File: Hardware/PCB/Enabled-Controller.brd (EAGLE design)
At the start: 54 x 71 mm, 19 parts, among them J2 HEADER_FEMALE-1X2, J3 QWIIC, U1 ITSYBITSY

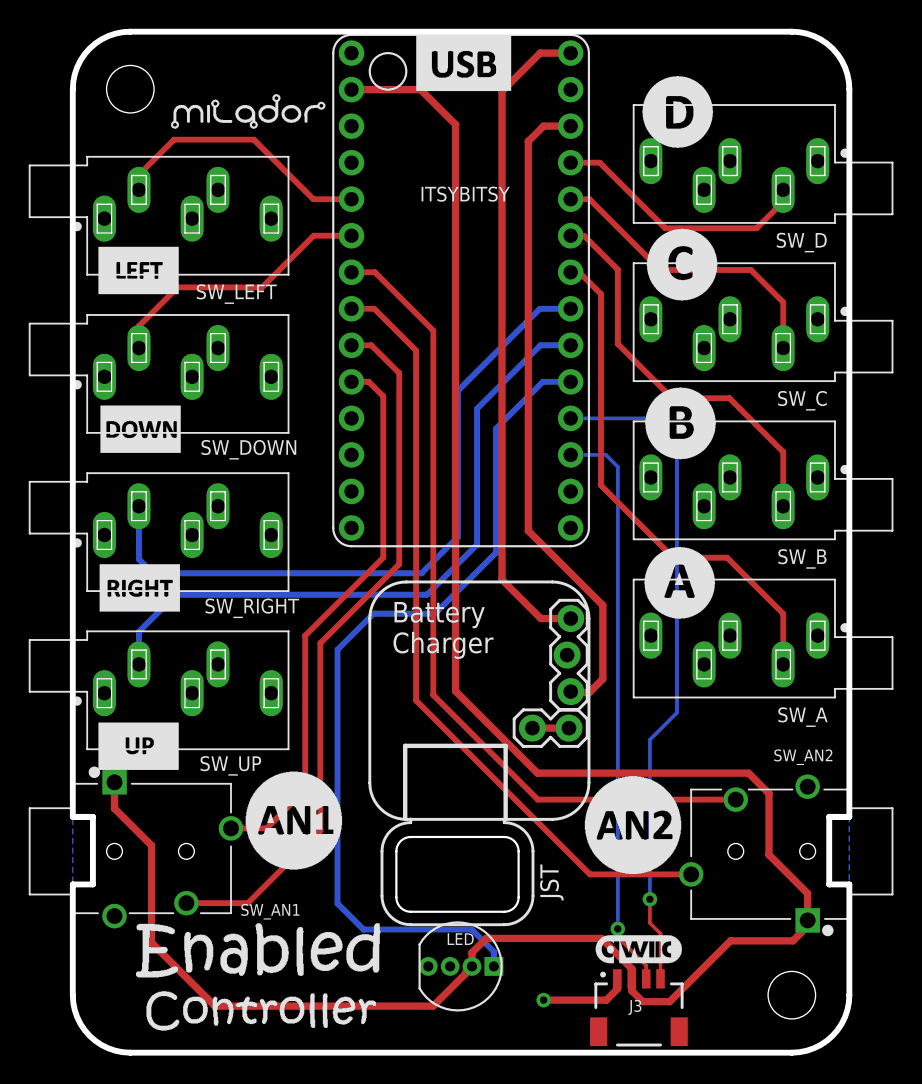
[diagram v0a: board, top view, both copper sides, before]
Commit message: Added updated PCB files
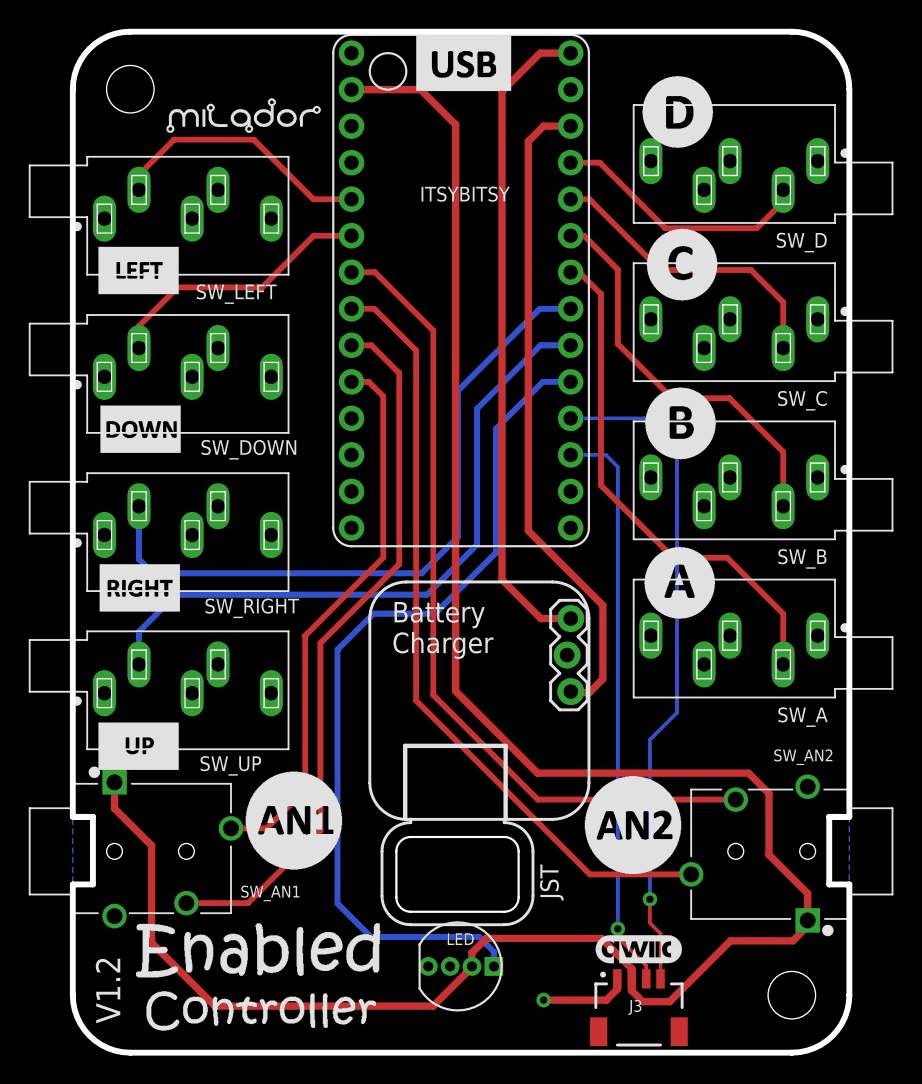
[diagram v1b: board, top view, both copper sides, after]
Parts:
- removed J2: HEADER_FEMALE-1X2, milador:HEADER_FEMALE-1X02
- removed U$1: MILADOR-LOGO-, milador:MILADOR_LOGO1
- added LABEL1: MILADOR-LOGO-, milador:MILADOR_LOGO1
- renumbered U$21 to LABEL2
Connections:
- removed net N$18: J2.1, J2.2
- net GND: now also J1.2, SW_A.3, SW_B.3, SW_C.3, SW_D.3, SW_DOWN.3, SW_LEFT.3, SW_RIGHT.3, SW_UP.3
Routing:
- net N$18: track 2.54 -> 0.00 mm
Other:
- board text added: "V1.2"
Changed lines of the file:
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@@
 <drawing>
 <settings>
-<setting alwaysvectorfont="yes"/>
+<setting alwaysvectorfont="no"/>
 <setting keepoldvectorfont="yes"/>
 <setting verticaltext="up"/>
@@
 <layer number="20" name="Dimension" color="15" fill="1" visible="yes" active="yes"/>
 <layer number="21" name="tPlace" color="7" fill="1" visible="yes" active="yes"/>
-<layer number="22" name="bPlace" color="7" fill="1" visible="yes" active="yes"/>
+<layer number="22" name="bPlace" color="7" fill="1" visible="no" active="yes"/>
 <layer number="23" name="tOrigins" color="15" fill="1" visible="yes" active="yes"/>
 <layer number="24" name="bOrigins" color="15" fill="1" visible="yes" active="yes"/>
@@
 </layers>
 <board>
-<fusionsync huburn="a.cGVyc29uYWw6dWUyYWQxOTI2" projecturn="a.cGVyc29uYWw6dWUyYWQxOTI2IzIwMjAwODAxMzIwMTk3MTgx" f3durn="urn:adsk.wipprod:dm.lineage:0P3WCUaEQdKCa3VO5MvKcA" pcbguid="" lastpulledtime="" lastsyncedchangeguid="" latestrevisionid="d0e29ba4-d4c4-4277-8ff9-67c412f5de14" lastsyncedrevisionid="d0e29ba4-d4c4-4277-8ff9-67c412f5de14" lastboardhashguid="a98b978c-a84a-6d7b-aef6-eb2471a3cdfa" lastpushedtime="2021-06-05T22:54:26Z" linktopcb3d="true"/>
+<fusionsync huburn="a.cGVyc29uYWw6dWUyYWQxOTI2" projecturn="a.cGVyc29uYWw6dWUyYWQxOTI2IzIwMjAwODAxMzIwMTk3MTgx" f3durn="urn:adsk.wipprod:dm.lineage:0P3WCUaEQdKCa3VO5MvKcA" pcbguid="" lastpulledtime="" lastsyncedchangeguid="" latestrevisionid="83d8bdd9-ecd9-4150-ad09-6a1a40ea1fac" lastsyncedrevisionid="83d8bdd9-ecd9-4150-ad09-6a1a40ea1fac" lastboardhashguid="a26c7ad2-ae5e-e781-a83e-f818fcadd8db" lastpushedtime="2021-06-10T00:37:29Z" linktopcb3d="true"/>
 <plain>
 <wire x1="4" y1="0" x2="50" y2="0" width="0.4064" layer="20"/>
@@
 <wire x1="30" y1="16" x2="30" y2="16.25" width="0.2" layer="21"/>
 <text x="33.782" y="10.668" size="1.27" layer="21" rot="R90">JST</text>
+<text x="3.302" y="2.032" size="1.6764" layer="21" ratio="20" rot="R90">V1.2</text>
 </plain>
 <attributes>
@@
 </element>
 <element name="SW_AN1" library="MMC Eagle" library_urn="urn:adsk.eagle:library:13126479" package="CUI_SJ-43514" package3d_urn="urn:adsk.eagle:package:22282311/2" value="SJ-43514" x="5.5" y="14" smashed="yes">
-<attribute name="NAME" x="11.648" y="9.5238" size="0.8128" layer="25"/>
+<attribute name="NAME" x="11.648" y="10.7938" size="0.8128" layer="25"/>
 </element>
 <element name="SW_AN2" library="MMC Eagle" library_urn="urn:adsk.eagle:library:13126479" package="CUI_SJ-43514" package3d_urn="urn:adsk.eagle:package:22282311/2" value="SJ-43514" x="48.5" y="14" smashed="yes" rot="R180">
@@
 <attribute name="VALUE" x="32.468" y="31.46" size="0.6096" layer="27" font="vector" ratio="20" rot="R270"/>
 </element>
-<element name="J2" library="milador" library_urn="urn:adsk.eagle:library:12595918" package="HEADER_FEMALE-1X02" package3d_urn="urn:adsk.eagle:package:27250301/1" value="HEADER_FEMALE-1X2" x="31.96" y="22.57" smashed="yes"/>
-<element name="U$1" library="milador" library_urn="urn:adsk.eagle:library:12595918" package="MILADOR_LOGO1" package3d_urn="urn:adsk.eagle:package:28431737/1" value="MILADOR-LOGO-" x="12.319" y="64.2874" smashed="yes"/>
-<element name="U$21" library="SparkFun-Aesthetics" package="QWIIC_6MM" value="" x="39.3954" y="7.1882" smashed="yes"/>
+<element name="LABEL1" library="milador" library_urn="urn:adsk.eagle:library:12595918" package="MILADOR_LOGO1" package3d_urn="urn:adsk.eagle:package:28431737/1" value="MILADOR-LOGO-" x="12" y="64" smashed="yes"/>
+<element name="LABEL2" library="SparkFun-Aesthetics" package="QWIIC_6MM" value="" x="39.3954" y="7.1882" smashed="yes"/>
 </elements>
 <signals>
@@
 <wire x1="37.87" y1="4.4182" x2="37.87" y2="5.133340625" width="0.508" layer="1"/>
 <wire x1="37.1094" y1="3.6576" x2="37.87" y2="4.4182" width="0.508" layer="1"/>
+<contactref element="SW_UP" pad="3"/>
+<contactref element="SW_RIGHT" pad="3"/>
+<contactref element="SW_A" pad="3"/>
+<contactref element="SW_B" pad="3"/>
+<contactref element="SW_C" pad="3"/>
+<contactref element="SW_D" pad="3"/>
+<contactref element="SW_DOWN" pad="3"/>
+<contactref element="SW_LEFT" pad="3"/>
+<contactref element="J1" pad="2"/>
 </signal>
 <signal name="+3V3">
@@
 <wire x1="32.6851" y1="46.65" x2="34.62" y2="46.65" width="0.4064" layer="16"/>
 <wire x1="29.28" y1="6" x2="29.28" y2="7.02" width="0.4064" layer="16"/>
-<wire x1="29.28" y1="7.02" x2="27.74" y2="8.56" width="0.4064" layer="16"/>
-<wire x1="27.74" y1="8.56" x2="20.22" y2="8.56" width="0.4064" layer="16"/>
-<wire x1="20.22" y1="8.56" x2="18.41" y2="10.37" width="0.4064" layer="16"/>
+<wire x1="29.28" y1="7.02" x2="28.248" y2="8.052" width="0.4064" layer="16"/>
+<wire x1="28.248" y1="8.052" x2="20.728" y2="8.052" width="0.4064" layer="16"/>
+<wire x1="20.728" y1="8.052" x2="18.41" y2="10.37" width="0.4064" layer="16"/>
 <wire x1="29.43321875" y1="34.76945625" x2="29.43321875" y2="43.39811875" width="0.4064" layer="16"/>
 <wire x1="29.43321875" y1="43.39811875" x2="32.6851" y2="46.65" width="0.4064" layer="16"/>
@@
 <wire x1="29.845" y1="32.893" x2="32.548" y2="30.19" width="0.508" layer="1"/>
 </signal>
-<signal name="N$18">
-<contactref element="J2" pad="2"/>
-<contactref element="J2" pad="1"/>
-<wire x1="34.5" y1="22.57" x2="31.96" y2="22.57" width="0.508" layer="1"/>
-</signal>
 </signals>
